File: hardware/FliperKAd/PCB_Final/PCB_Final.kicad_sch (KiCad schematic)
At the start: 54 parts, among them J101 Conn_01x02, J102 Conn_ST_STDC14, J103 Conn_01x04, J104 Conn_01x04, J105 Conn_01x06, J106 Conn_01x03, SW101 SW_Push, SW102 SW_Push, SW103 SW_Push, U104 STM32G431KBTx

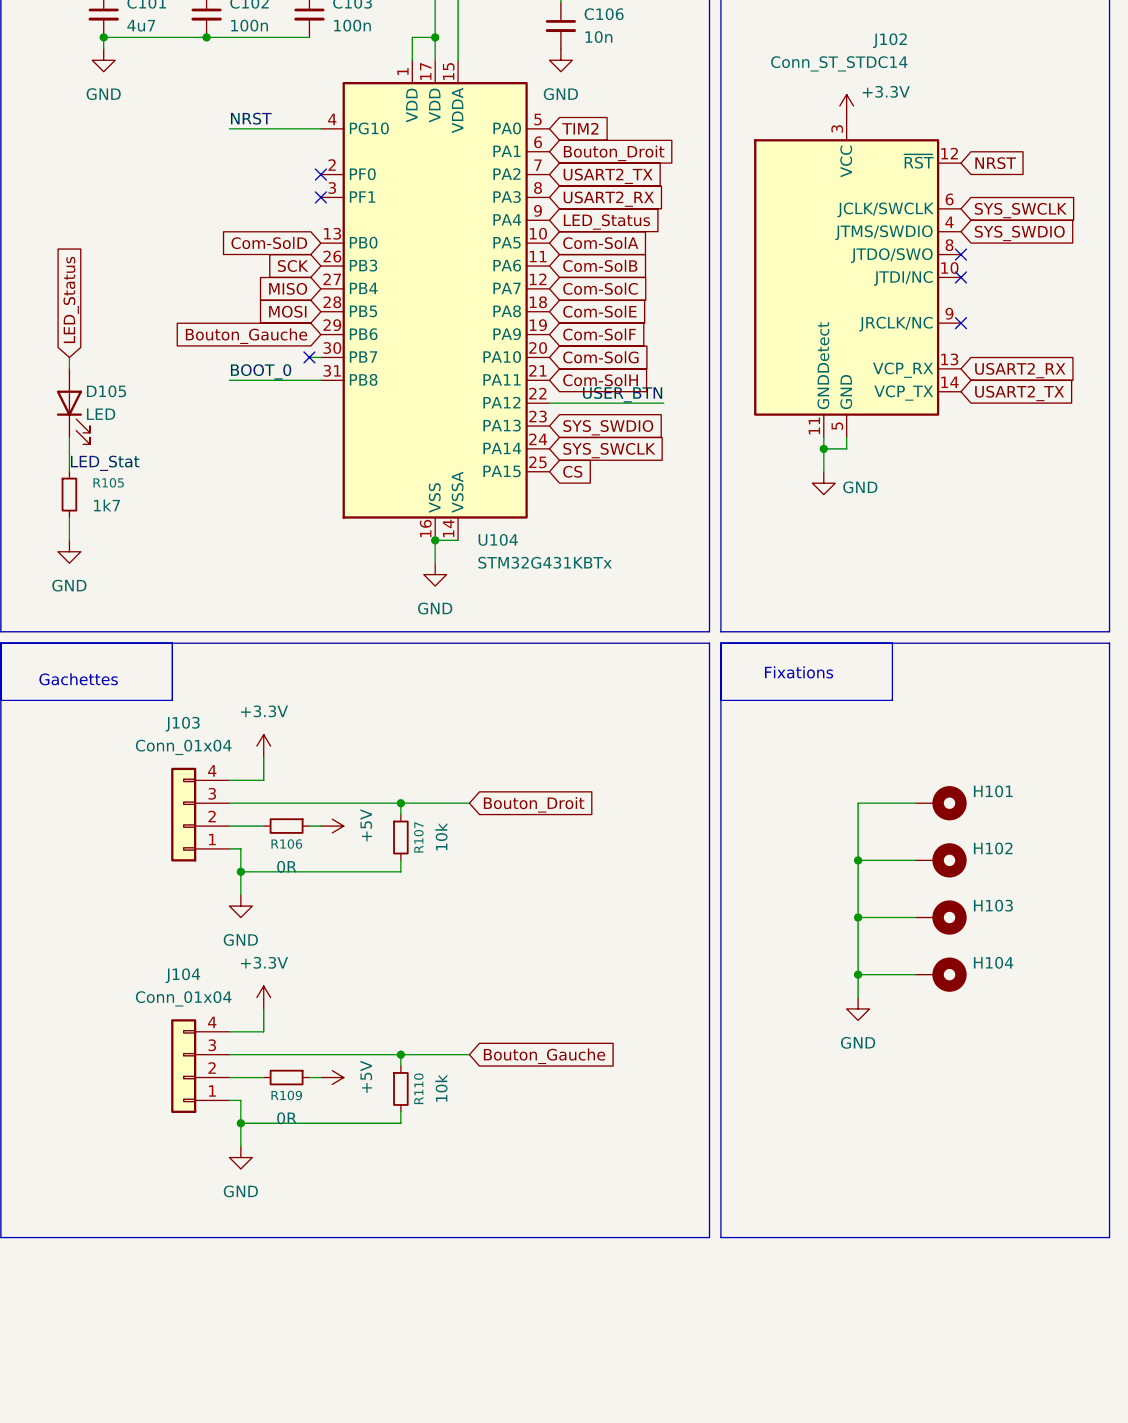
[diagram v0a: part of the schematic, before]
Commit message: pour le compte rendu
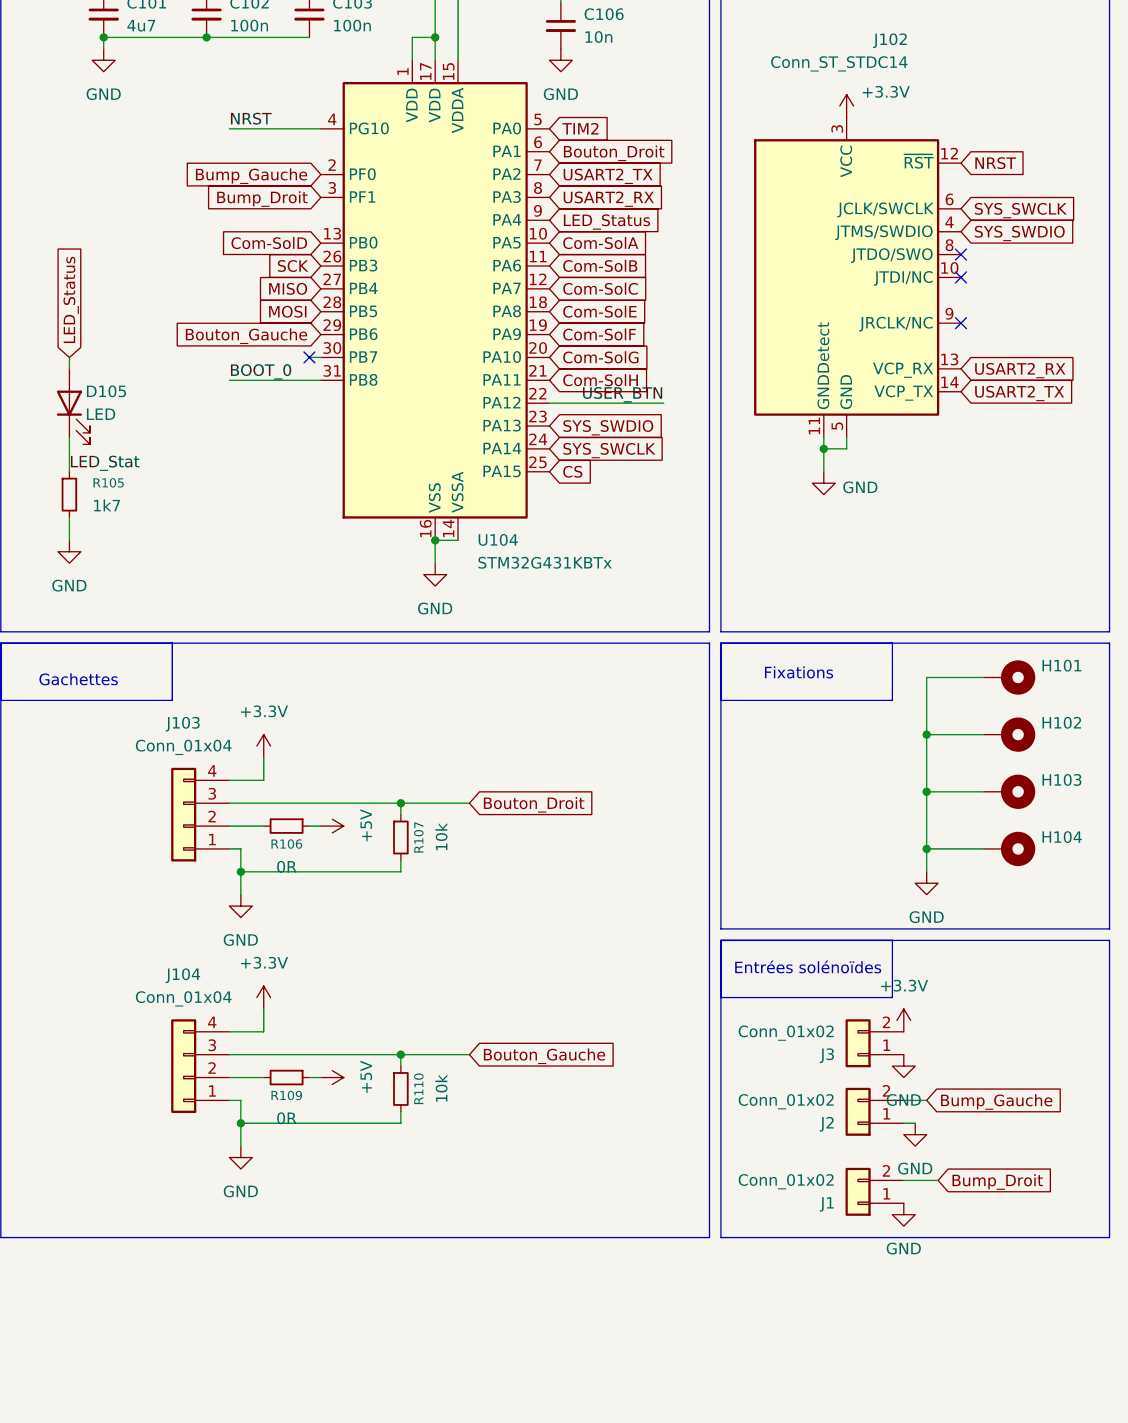
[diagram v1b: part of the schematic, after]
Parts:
- added J1, J2, J3: Conn_01x02, Connector_JST:JST_PH_B2B-PH-K_1x02_P2.00mm_Vertical, symbol Connector_Generic:Conn_01x02
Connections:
- net +3.3V: now also J3.2 (Pin_2)
- net GND: now also J1.1 (Pin_1), J2.1 (Pin_1), J3.1 (Pin_1)
- net Bump_Gauche: now reaches U104.2 (PF0)
- net Bump_Gauche: now also J2.2 (Pin_2)
- net Bump_Droit: now reaches U104.3 (PF1)
- net Bump_Droit: now also J1.2 (Pin_2)
- no-connect marks 6 -> 4
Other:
- note added: "Entrées solénoïdes"
- moved on the sheet: H101, H102, H103, H104
